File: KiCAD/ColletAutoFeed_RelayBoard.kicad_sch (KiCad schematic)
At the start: 3 parts, among them J1 1761685-6, J2 690367190472, U1 ProS3

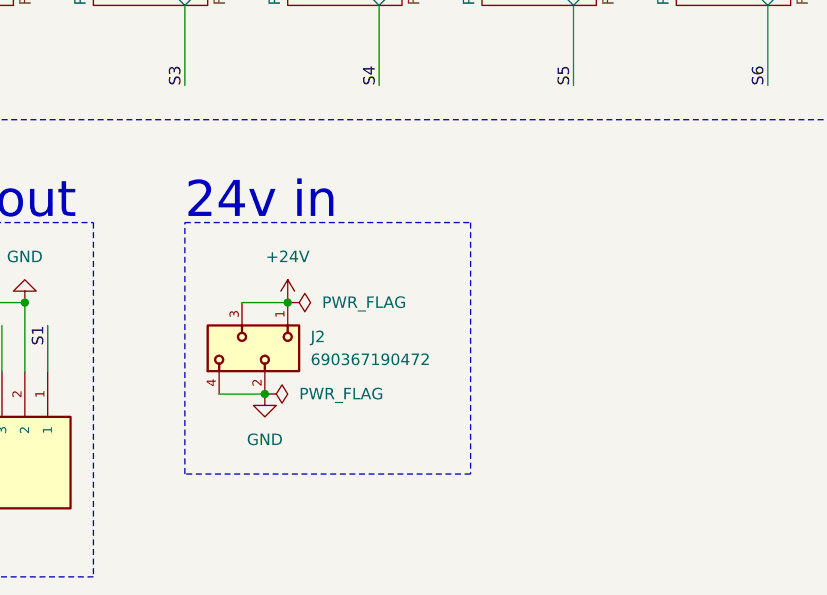
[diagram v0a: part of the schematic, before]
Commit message: Started PCB layout
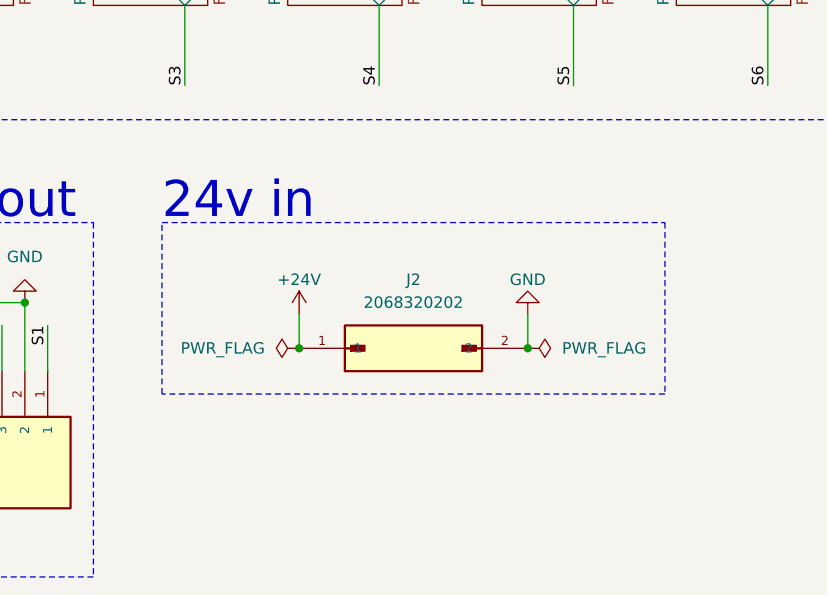
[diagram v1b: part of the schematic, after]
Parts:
- removed J2: 690367190472, WR-MM:690367190472, symbol WR-MM-04:690367190472
- added J2: 2068320202, Molex 206832-0202:MOLEX_2068320202, symbol Molex 206832-0202:2068320202
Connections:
- net +24V: now also J2.1
- net GND: now also J2.2
